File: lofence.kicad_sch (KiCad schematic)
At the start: 58 parts, among them J1 Fence+, J2 Fence-, J3 ISP, J4 DEBUG LA, J5 DEBUG LED, J6 DEBUG MCU, SW1 RESET, U1 TLV9062, U3 ATmega328PB-AU, U4 LA66, U5 MCP1253-33X50I/MS, Y1 32768 Hz

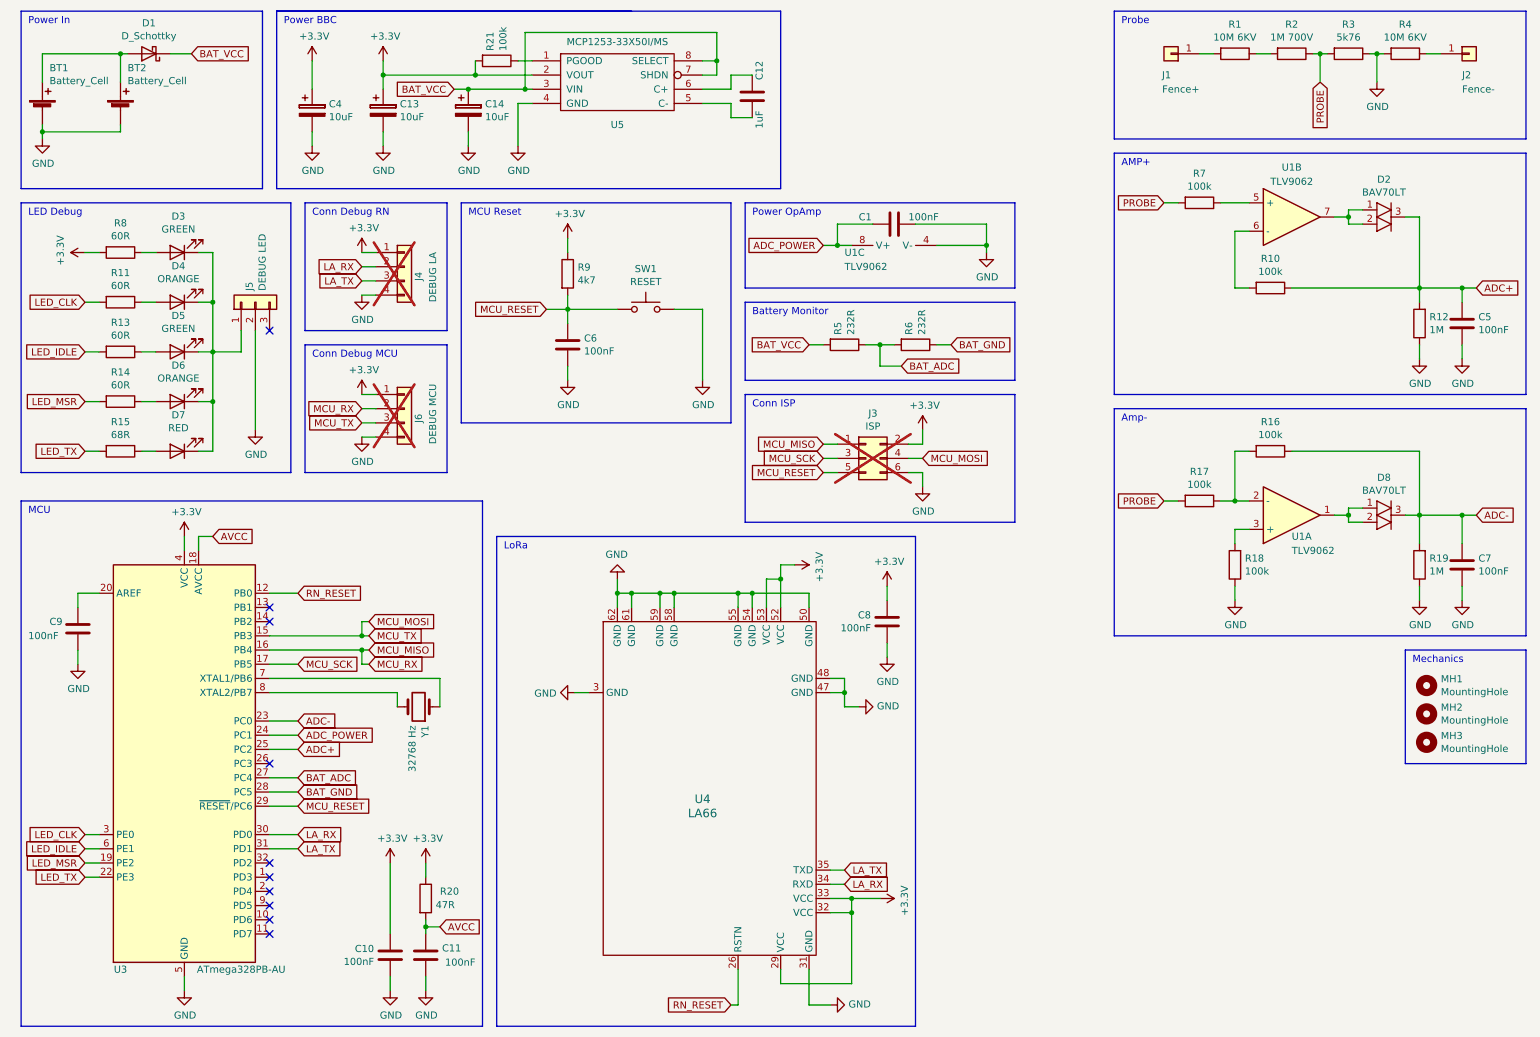
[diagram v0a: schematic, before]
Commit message: update layout, prepared for production
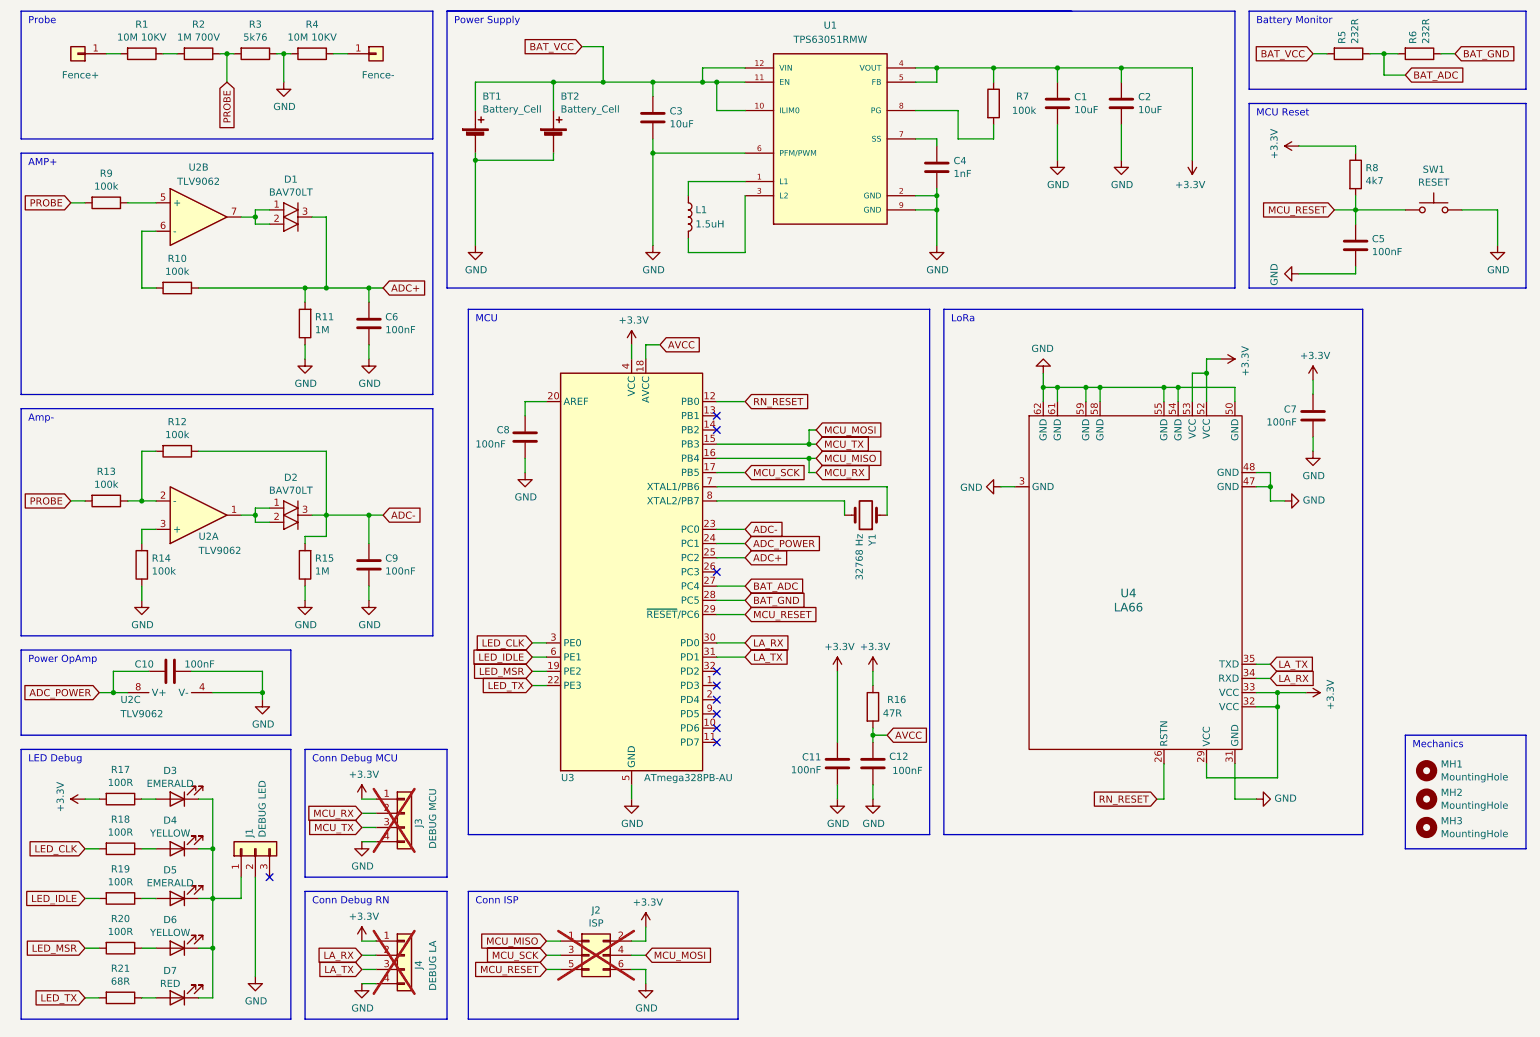
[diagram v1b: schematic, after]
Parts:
- removed C12: 1uF, Capacitor_SMD:C_0805_2012Metric_Pad1.18x1.45mm_HandSolder, symbol Device:C
- removed D1: D_Schottky, Diode_SMD:D_SMA_Handsoldering, symbol Device:D_Schottky
- removed U5: MCP1253-33X50I/MS, Package_SO:MSOP-8_3x3mm_P0.65mm, symbol ALITECS:MCP125x
- added C4: 1nF, Capacitor_SMD:C_0805_2012Metric_Pad1.18x1.45mm_HandSolder, symbol Device:C
- added L1: 1.5uH, Inductor_SMD:L_1008_2520Metric_Pad1.43x2.20mm_HandSolder, symbol Device:L
- added U1: TPS63051RMW, ALITECS:TPS63051RMW, symbol ALITECS:TPS63051RMW
- C1: renamed from C13; footprint Capacitor_SMD:C_1206_3216Metric_Pad1.33x1.80mm_HandSolder -> Capacitor_SMD:C_0805_2012Metric_Pad1.18x1.45mm_HandSolder; symbol lofence-rescue:CP-Device -> Device:C
- C2: renamed from C14; footprint Capacitor_SMD:C_1206_3216Metric_Pad1.33x1.80mm_HandSolder -> Capacitor_SMD:C_0805_2012Metric_Pad1.18x1.45mm_HandSolder; symbol lofence-rescue:CP-Device -> Device:C
- C3: renamed from C4; footprint Capacitor_SMD:CP_Elec_4x5.4 -> Capacitor_SMD:C_0805_2012Metric_Pad1.18x1.45mm_HandSolder; symbol lofence-rescue:CP-Device -> Device:C; JLCPCB Part # C4747969 -> C13585
- D1: renamed from D2; JLCPCB Rotation Offset (none) -> 180
- D2: renamed from D8; JLCPCB Rotation Offset (none) -> 180
- D3, D5: value GREEN -> EMERALD; JLCPCB Part # C84257 -> C2297
- D4, D6: value ORANGE -> YELLOW; JLCPCB Part # C84262 -> C2296
- MH1, MH2, MH3: footprint MountingHole:MountingHole_2.7mm_M2.5 -> MountingHole:MountingHole_3.2mm_M3_DIN965_Pad
- R1, R4: value 10M 6KV -> 10M 10KV; TME Order # (none) -> VR68000001005JAC00
- R10: footprint Resistor_SMD:R_0805_2012Metric_Pad1.20x1.40mm_HandSolder -> Resistor_SMD:R_0603_1608Metric_Pad0.98x0.95mm_HandSolder; JLCPCB Part # C149504 -> (none)
- R11: renamed from R12; footprint Resistor_SMD:R_0805_2012Metric_Pad1.20x1.40mm_HandSolder -> Resistor_SMD:R_0603_1608Metric_Pad0.98x0.95mm_HandSolder; JLCPCB Part # C17514 -> (none)
- R12: renamed from R16; footprint Resistor_SMD:R_0805_2012Metric_Pad1.20x1.40mm_HandSolder -> Resistor_SMD:R_0603_1608Metric_Pad0.98x0.95mm_HandSolder; JLCPCB Part # C149504 -> (none)
- R13: renamed from R17; footprint Resistor_SMD:R_0805_2012Metric_Pad1.20x1.40mm_HandSolder -> Resistor_SMD:R_0603_1608Metric_Pad0.98x0.95mm_HandSolder; JLCPCB Part # C149504 -> (none)
- R14: renamed from R18; footprint Resistor_SMD:R_0805_2012Metric_Pad1.20x1.40mm_HandSolder -> Resistor_SMD:R_0603_1608Metric_Pad0.98x0.95mm_HandSolder; JLCPCB Part # C149504 -> (none)
- R15: renamed from R19; footprint Resistor_SMD:R_0805_2012Metric_Pad1.20x1.40mm_HandSolder -> Resistor_SMD:R_0603_1608Metric_Pad0.98x0.95mm_HandSolder; JLCPCB Part # C17514 -> (none)
- R16: renamed from R20; footprint Resistor_SMD:R_0805_2012Metric_Pad1.20x1.40mm_HandSolder -> Resistor_SMD:R_0603_1608Metric_Pad0.98x0.95mm_HandSolder; JLCPCB Part # C17714 -> (none)
- R17: renamed from R8; value 60R -> 100R; footprint Resistor_SMD:R_0805_2012Metric_Pad1.20x1.40mm_HandSolder -> Resistor_SMD:R_0603_1608Metric_Pad0.98x0.95mm_HandSolder; JLCPCB Part # C2767521 -> (none)
- R18: renamed from R11; value 60R -> 100R; footprint Resistor_SMD:R_0805_2012Metric_Pad1.20x1.40mm_HandSolder -> Resistor_SMD:R_0603_1608Metric_Pad0.98x0.95mm_HandSolder; JLCPCB Part # C2767521 -> (none)
- R19: renamed from R13; value 60R -> 100R; footprint Resistor_SMD:R_0805_2012Metric_Pad1.20x1.40mm_HandSolder -> Resistor_SMD:R_0603_1608Metric_Pad0.98x0.95mm_HandSolder; JLCPCB Part # C2767521 -> (none)
- R20: renamed from R14; value 60R -> 100R; footprint Resistor_SMD:R_0805_2012Metric_Pad1.20x1.40mm_HandSolder -> Resistor_SMD:R_0603_1608Metric_Pad0.98x0.95mm_HandSolder; JLCPCB Part # C2767521 -> (none)
- R21: renamed from R15; footprint Resistor_SMD:R_0805_2012Metric_Pad1.20x1.40mm_HandSolder -> Resistor_SMD:R_0603_1608Metric_Pad0.98x0.95mm_HandSolder; JLCPCB Part # C17802 -> (none)
- R5, R6: footprint Resistor_SMD:R_0805_2012Metric_Pad1.20x1.40mm_HandSolder -> Resistor_SMD:R_0603_1608Metric_Pad0.98x0.95mm_HandSolder; JLCPCB Part # C5200550 -> C22913
- R7: renamed from R21; footprint Resistor_SMD:R_0805_2012Metric_Pad1.20x1.40mm_HandSolder -> Resistor_SMD:R_0603_1608Metric_Pad0.98x0.95mm_HandSolder; JLCPCB Part # C149504 -> (none)
- R8: renamed from R9; footprint Resistor_SMD:R_0805_2012Metric_Pad1.20x1.40mm_HandSolder -> Resistor_SMD:R_0603_1608Metric_Pad0.98x0.95mm_HandSolder; JLCPCB Part # C17673 -> (none)
- R9: renamed from R7; footprint Resistor_SMD:R_0805_2012Metric_Pad1.20x1.40mm_HandSolder -> Resistor_SMD:R_0603_1608Metric_Pad0.98x0.95mm_HandSolder; JLCPCB Part # C149504 -> (none)
- U2: renamed from U1; JLCPCB Rotation Offset (none) -> -90
- U3: JLCPCB Rotation Offset (none) -> -90
- renumbered C1 to C10, C10 to C11, C11 to C12, C6 to C5, C5 to C6, C8 to C7, C9 to C8, C7 to C9, J5 to J1, J1 to J101, J2 to J102, J3 to J2, J6 to J3
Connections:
- net +3V3: now also C2.1, R7.1, U1.4 (VOUT), U1.5 (FB); no longer C3.1, R7.2
- net BAT_VCC: now also BT1.1 (+), BT2.1 (+), C3.1, U1.10 (ILIM0), U1.11 (EN), U1.12 (VIN); no longer C2.1
- net GND: now also C4.2, U1.2 (GND), U1.6 (PFM/PWM), U1.9 (GND)
- new net: R7.2, U1.8 (PG)
- new net: L1.1, U1.1 (L1)
- new net: L1.2, U1.3 (L2)
- new net: C4.1, U1.7 (SS)
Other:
- note added: "Power Supply"
- note removed: "Power BBC"
- note removed: "Power In"
- moved on the sheet: BT1, BT2, C10, C11, C12, C5, C6, C7, C8, C9, D1, D2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
